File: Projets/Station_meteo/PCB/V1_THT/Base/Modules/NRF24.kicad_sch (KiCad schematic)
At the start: 7 parts, among them U7 NRF24L01_Breakout

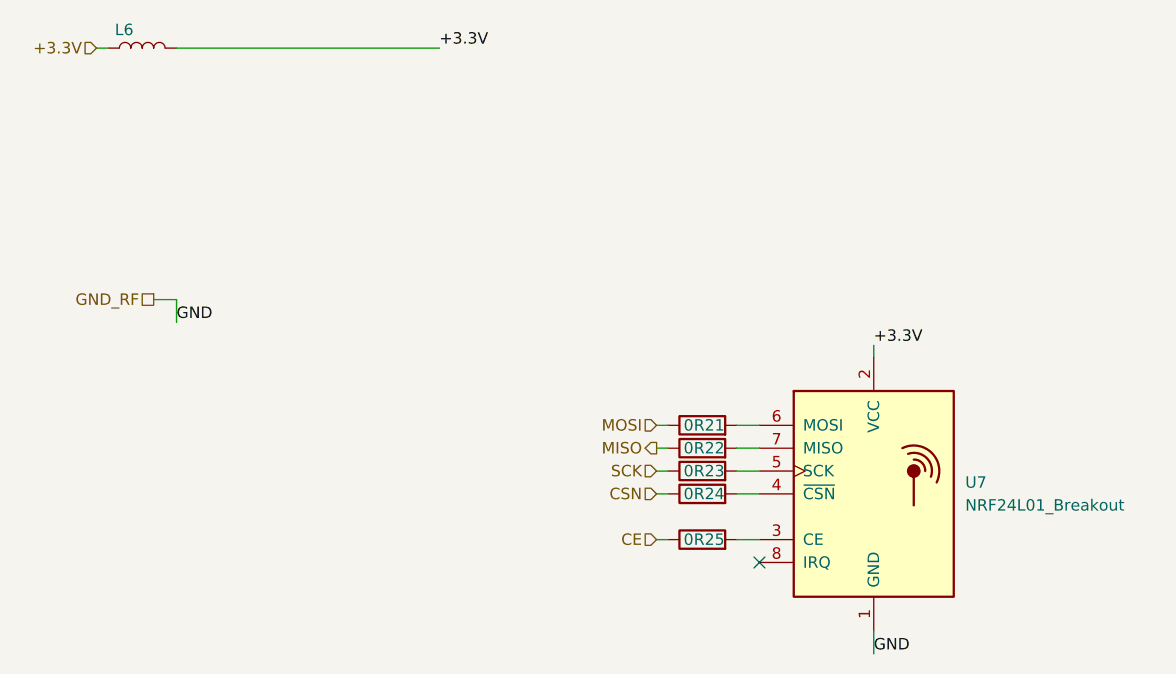
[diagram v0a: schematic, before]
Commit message: Update
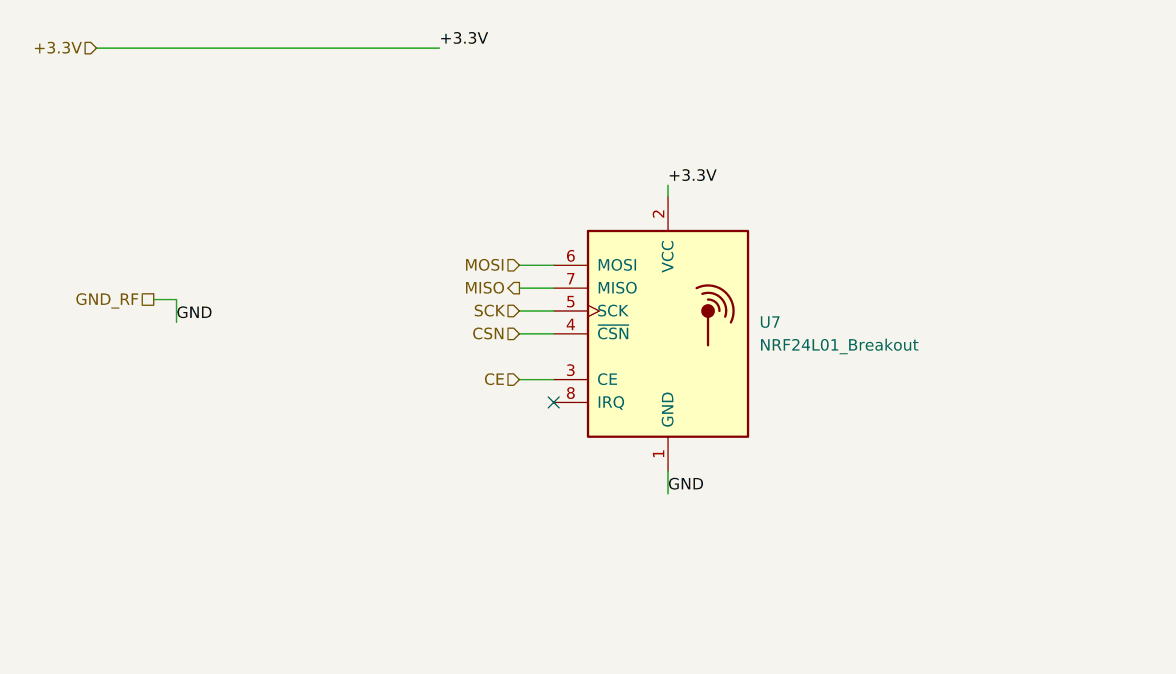
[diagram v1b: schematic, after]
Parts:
- removed L6: MPZ1608S101ATAH0, Inductor_SMD:L_0603_1608Metric, symbol Device:L
- removed R21, R22, R23, R24, R25: 0, Resistor_SMD:R_0603_1608Metric, symbol Device:R
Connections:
- net CE: now also U7.3 (CE)
- net CSN: now also U7.4 (~{CSN})
- net MISO: now also U7.7 (MISO)
- net MOSI: now also U7.6 (MOSI)
- net SCK: now also U7.5 (SCK)
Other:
- moved on the sheet: U7

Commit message: Update Weather station
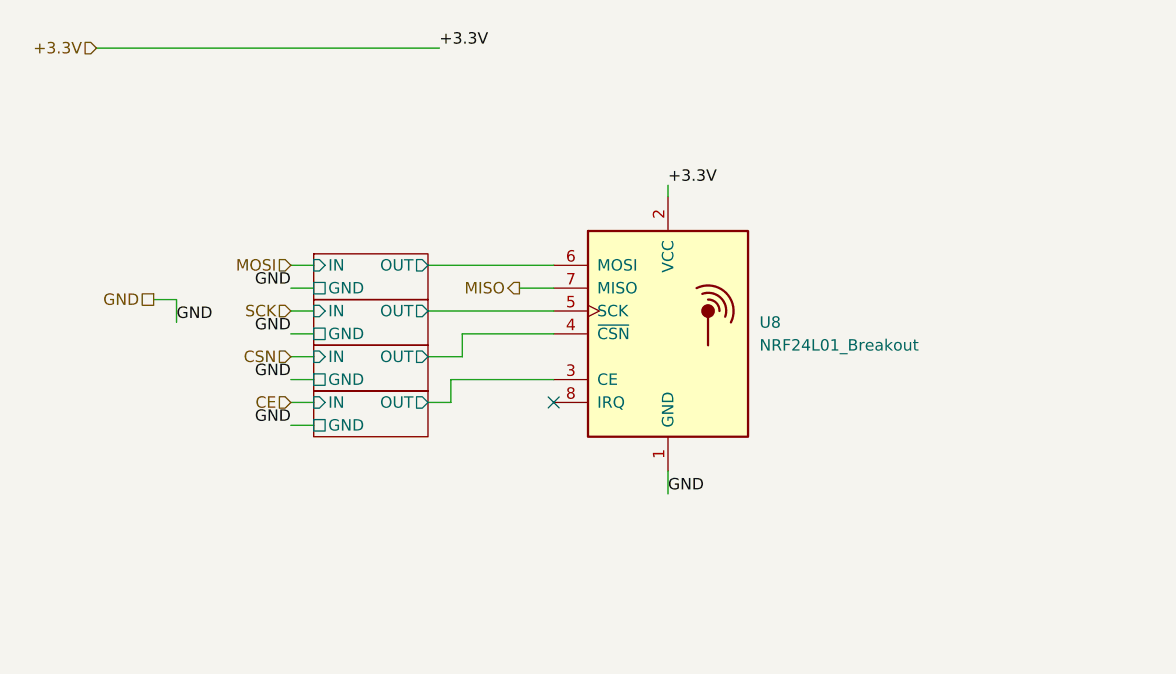
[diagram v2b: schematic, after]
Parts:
- renumbered U7 to U8
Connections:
- net CE: no longer U8.3 (CE)
- net CSN: no longer U8.4 (~{CSN})
- net MOSI: no longer U8.6 (MOSI)
- net SCK: no longer U8.5 (SCK)
- net GND_RF renamed GND
- new net Bridge/OUT: U8.5 (SCK)
- new net Bridge1/OUT: U8.6 (MOSI)
- new net Bridge2/OUT: U8.4 (~{CSN})
- new net Bridge3/OUT: U8.3 (CE)
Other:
- added sheet Bridge (Bridge.kicad_sch)
- added sheet Bridge1 (Bridge.kicad_sch)
- added sheet Bridge2 (Bridge.kicad_sch)
- added sheet Bridge3 (Bridge.kicad_sch)

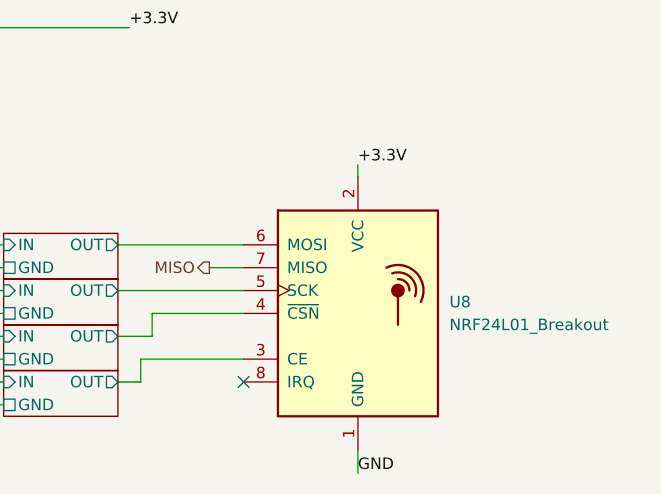
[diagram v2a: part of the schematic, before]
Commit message: Update
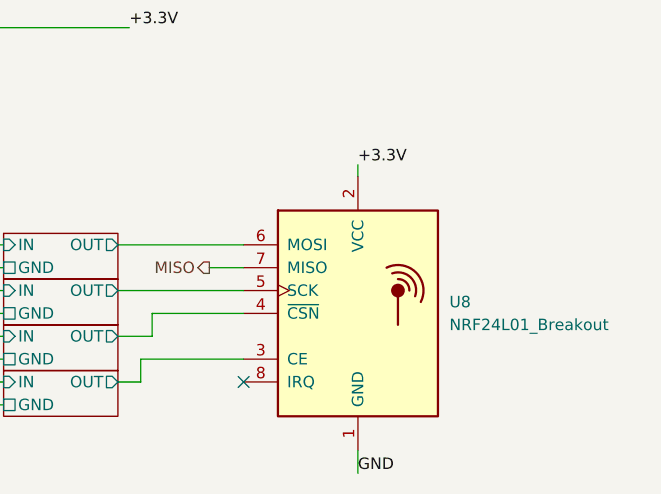
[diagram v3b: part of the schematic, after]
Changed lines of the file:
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@@
 (kicad_sch
-	(version 20231120)
+	(version 20250114)
 	(generator "eeschema")
-	(generator_version "8.0")
+	(generator_version "9.0")
 	(paper "A5")
 	(title_block
@@
 		(at 68.58 59.69)
 		(size 12.7 5.08)
+		(exclude_from_sim no)
+		(in_bom yes)
+		(on_board yes)
+		(dnp no)
 		(fields_autoplaced yes)
 		(stroke
@@
 		(at 68.58 74.93)
 		(size 12.7 5.08)
+		(exclude_from_sim no)
+		(in_bom yes)
+		(on_board yes)
+		(dnp no)
 		(fields_autoplaced yes)
 		(stroke
@@
 		(at 68.58 64.77)
 		(size 12.7 5.08)
+		(exclude_from_sim no)
+		(in_bom yes)
+		(on_board yes)
+		(dnp no)
 		(fields_autoplaced yes)
 		(stroke
@@
 		(at 68.58 69.85)
 		(size 12.7 5.08)
+		(exclude_from_sim no)
+		(in_bom yes)
+		(on_board yes)
+		(dnp no)
 		(fields_autoplaced yes)
 		(stroke
